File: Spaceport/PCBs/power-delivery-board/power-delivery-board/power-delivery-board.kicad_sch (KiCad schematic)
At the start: 40 parts, among them J1 Conn_01x07_Pin, U1 ADP5033ACBZ-5-R7, U2 TPS610986DSER, U3 TPS610986DSER

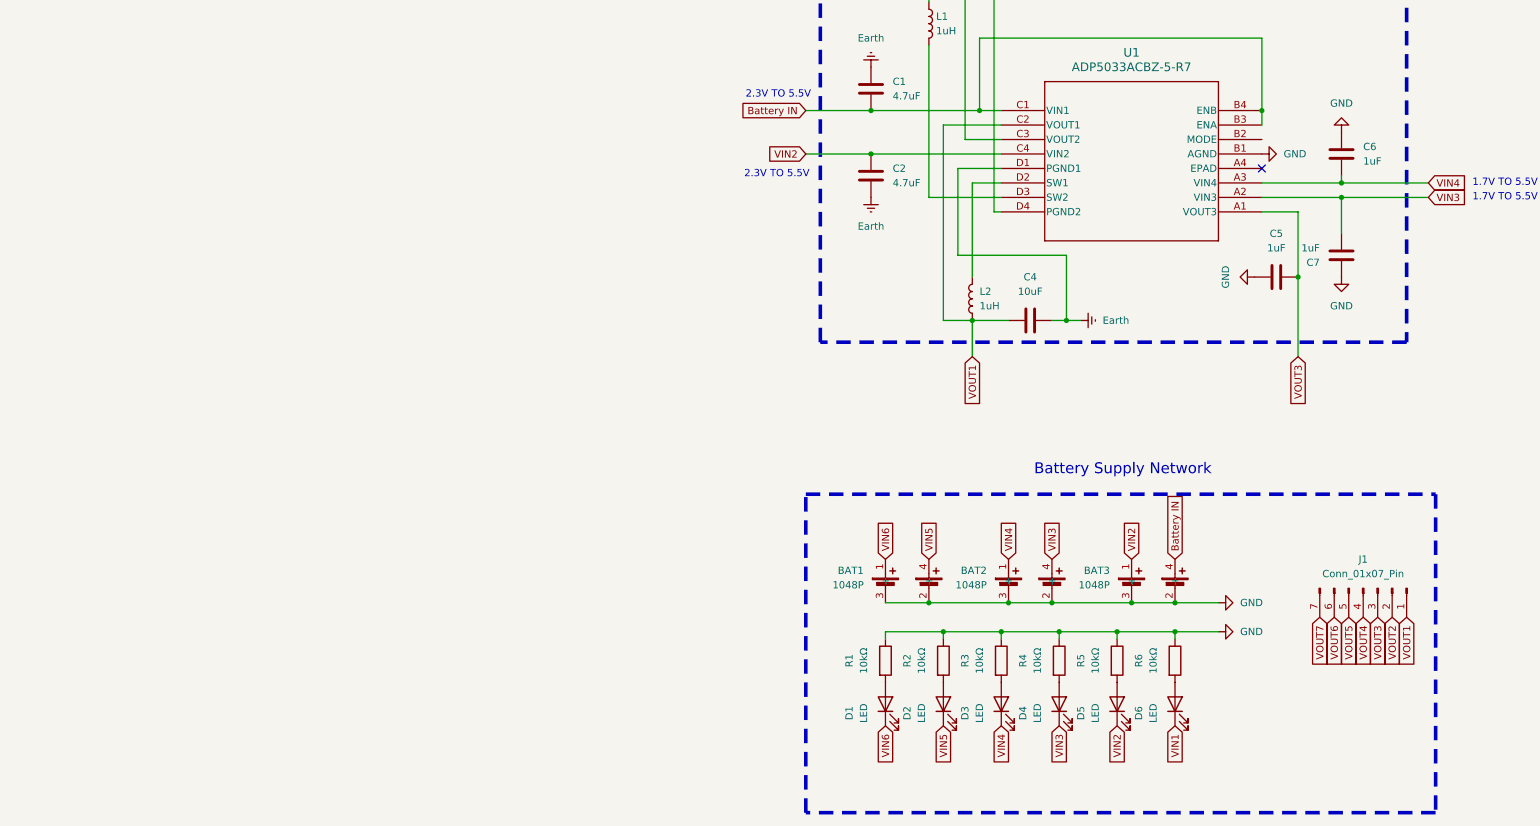
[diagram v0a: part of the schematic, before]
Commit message: Housekeeping File Updates
- Removed extra PCB file that somehow got onto the repo
- Updated PCB file with footprints
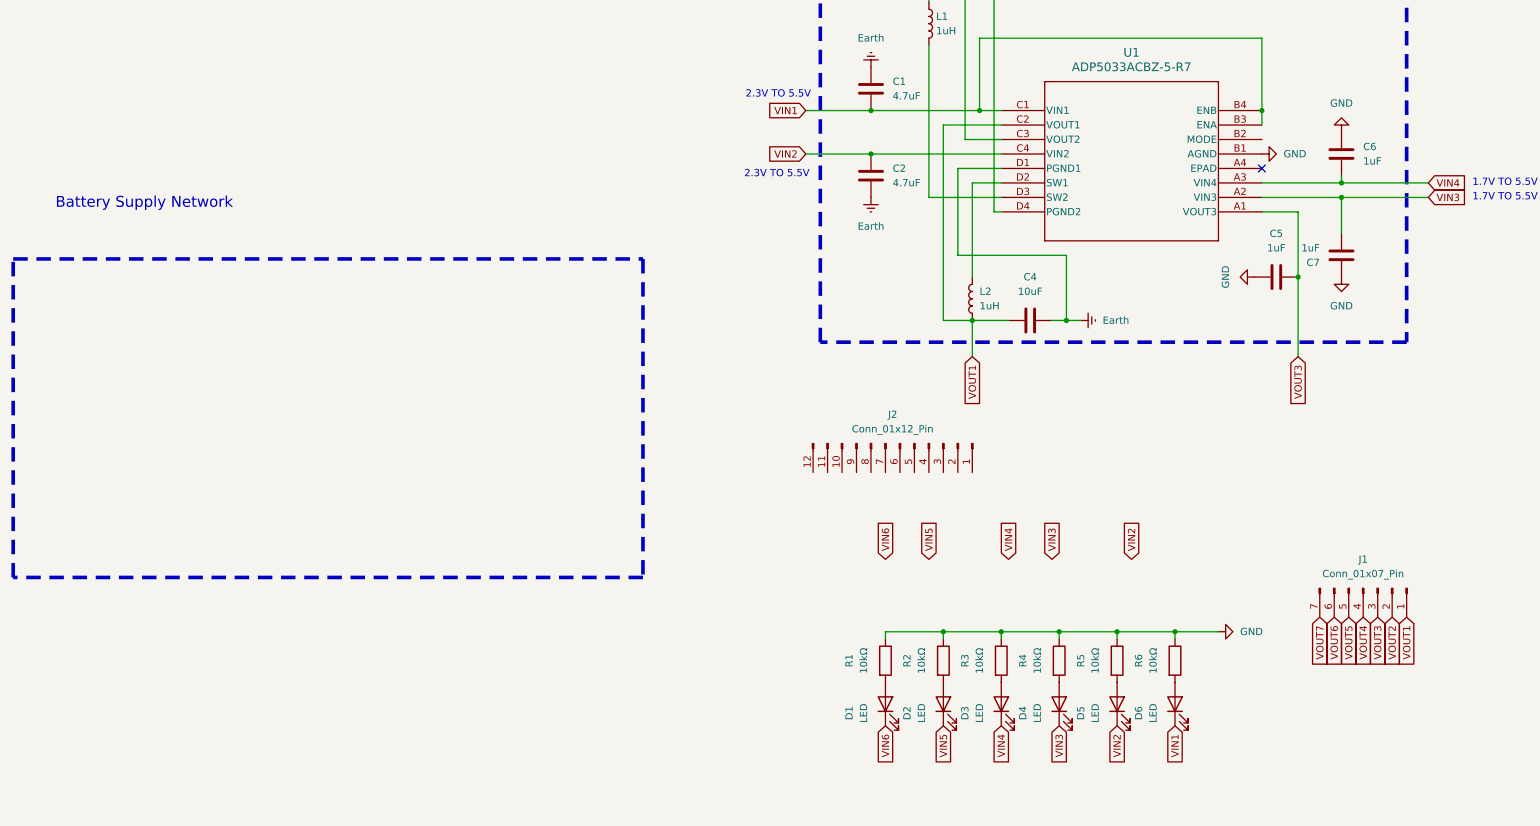
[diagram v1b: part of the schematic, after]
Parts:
- removed BAT1, BAT2, BAT3: 1048P, Avionics:BAT_1048P, symbol Avionics (1):1048P
- added J2: Conn_01x12_Pin, symbol Connector:Conn_01x12_Pin
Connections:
- net Battery IN is gone; now on net VIN1: C1.1, U1.B3 (ENA), U1.B4 (ENB), U1.C1 (VIN1)

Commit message: Add USB and 5V / 3A Topology
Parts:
- removed J2: Conn_01x12_Pin, symbol Connector:Conn_01x12_Pin
- added C10, C11, C12, C13: C, symbol Device:C
- added C8: 1uF, Capacitor_SMD:C_0805_2012Metric, symbol Device:C
- added C9: 4.7uF, symbol Device:C
- added D7, D8: LED, symbol Device:LED
- added J2: Conn_02x06_Row_Letter_Last, symbol Connector_Generic:Conn_02x06_Row_Letter_Last
- added L5: 2.2uH, symbol Device:L
- added P1: USB_C_Plug_USB2.0, symbol Connector:USB_C_Plug_USB2.0
- added R10, R9: 10kΩ, Resistor_SMD:R_0805_2012Metric, symbol Device:R
- added R11: 187kΩ, symbol Device:R
- added R12: 1MΩ, symbol Device:R
- added R13: R, symbol Device:R
- added R7: 1kΩ, symbol Device:R
- added R8: 5kΩ, symbol Device:R
- added U4: USBLC6-2P6, Package_TO_SOT_SMD:SOT-666, symbol Power_Protection:USBLC6-2P6
- added U4: BQ25185DLHR, WSON10_DLH_TEX, symbol Avionics (1):BQ25185DLHR
- added U5: LT8609AEDDM-5#TRPBF, SON50P300X300X85-11N-D, symbol Avionics (1):LT8609AEDDM-5#TRPBF
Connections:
- net GND: now also C12.1, C13.2, C8.1, C9.2, J2.1b (Pin_1b), J2.2b (Pin_2b), J2.3b (Pin_3b), J2.4b (Pin_4b), J2.5b (Pin_5b), J2.6b (Pin_6b), P1.A1 (GND), P1.A12 (GND), P1.B1 (GND), P1.B12 (GND), R10.1, R11.1, R13.2, R7.2, R8.2, R9.1, U4.2 (GND), U4.4 (/CE), U4.5 (GND), U5.11 (GND)
- net VIN1: now also J2.1a (Pin_1a)
- net VIN2: now also J2.2a (Pin_2a)
- net VIN3: now also J2.3a (Pin_3a)
- net VIN4: now also J2.4a (Pin_4a)
- net VIN5: now also J2.5a (Pin_5a)
- net VIN6: now also J2.6a (Pin_6a)
- new net: D7.2 (A), R9.2
- new net: P1.A7 (D-), U4.1 (I/O1)
- new net: P1.A6 (D+), U4.3 (I/O2)
- new net: R13.1, U5.4 (RT)
- new net: C13.1, U5.3 (INTVCC)
- new net: R8.1, U4.7 (ILIM/VSET)
- new net: D8.2 (A), R10.2
- new net: C10.2, U5.1 (BST)
- new net: C10.1, L5.2, U5.2 (SW)
- new net: R7.1, U4.8 (ISET)
- new net BAT+: U4.2 (BAT)
- new net D+: U4.4 (I/O2)
- new net D-: U4.6 (I/O1)
- new net FB: C11.1, R11.2, R12.1, U5.6 (FB)
- new net STAT1: D7.1 (K), U4.9 (STAT1)
- new net STAT2: D8.1 (K), U4.3 (STAT2)
- new net VBUS: C8.2, P1.A4 (VBUS), P1.A9 (VBUS), P1.B4 (VBUS), P1.B9 (VBUS), U4.10 (IN), U4.5 (VBUS)
- new net VIN7: C9.1, U5.9 (VIN)
- new net VOUT8: C11.2, C12.2, L5.1, R12.2
- no-connect marks 3 -> 8
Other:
- note added: "6V TO 40V"
- note added: "INPUT / OUTPUT"
- note added: "SOURCE THREE"
- note added: "STATUS LEDs"
- note added: "VOUT 8 5V 3A"
- note removed: "Battery Supply Network"
- moved on the sheet: C1, C2, C3, C4, C5, C6, C7, CBAT1, CBAT2, CIN1, CIN2, COUT1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

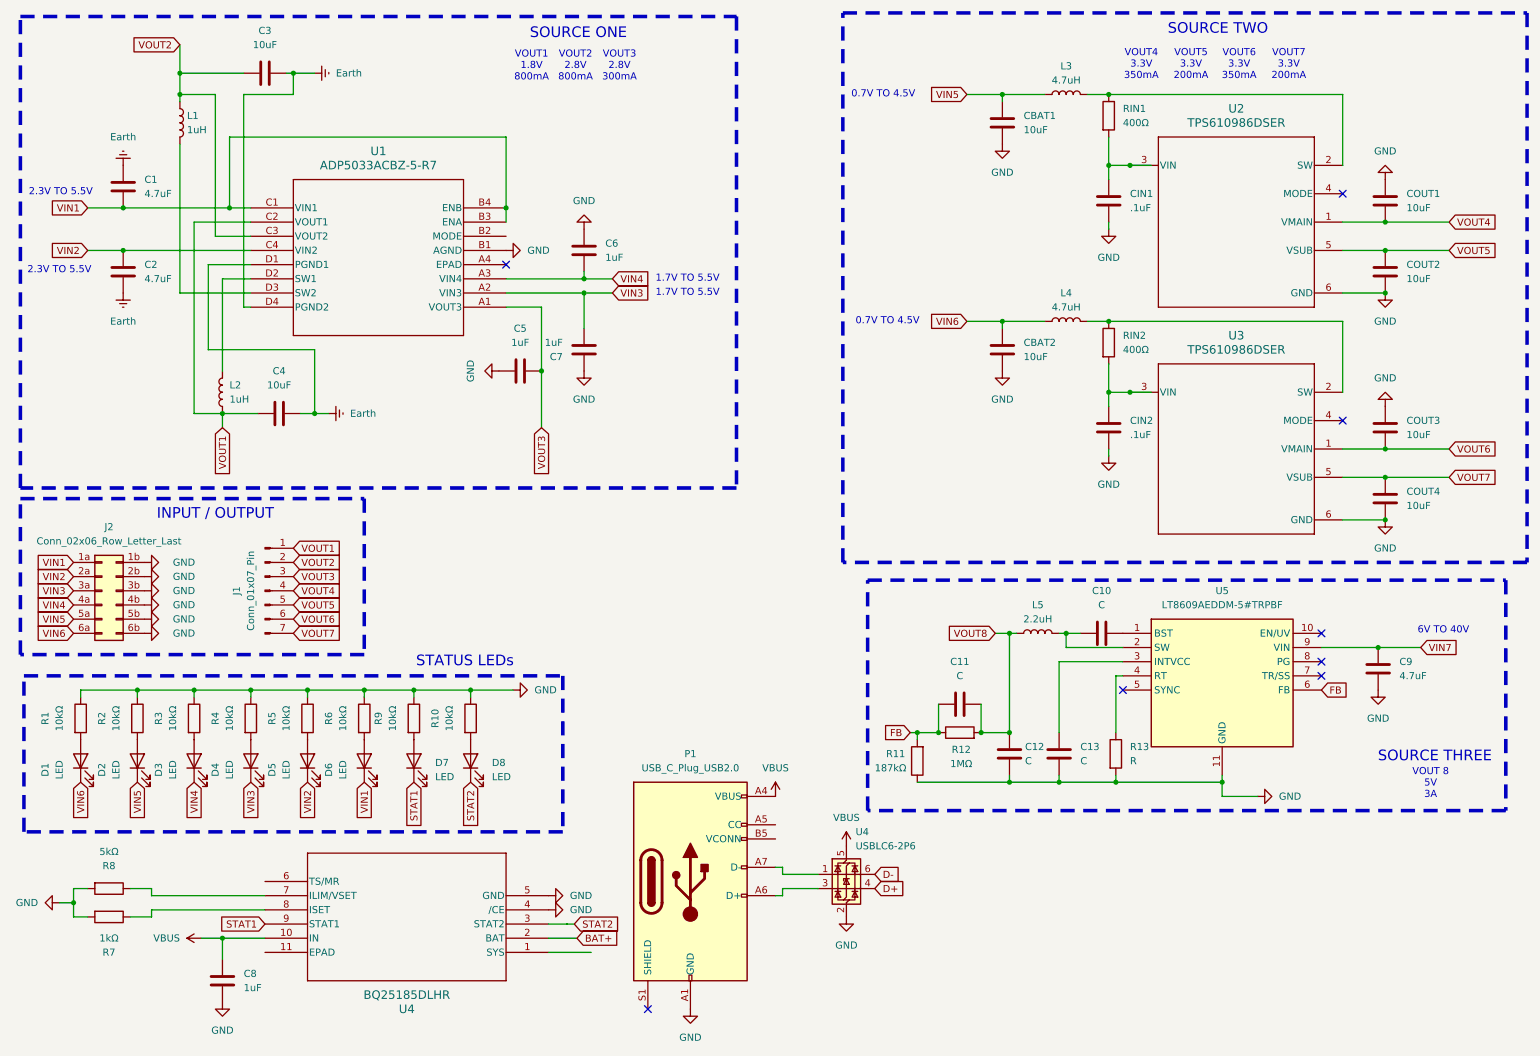
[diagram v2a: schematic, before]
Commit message: Schematic Updates. NOTE: ERC Fails
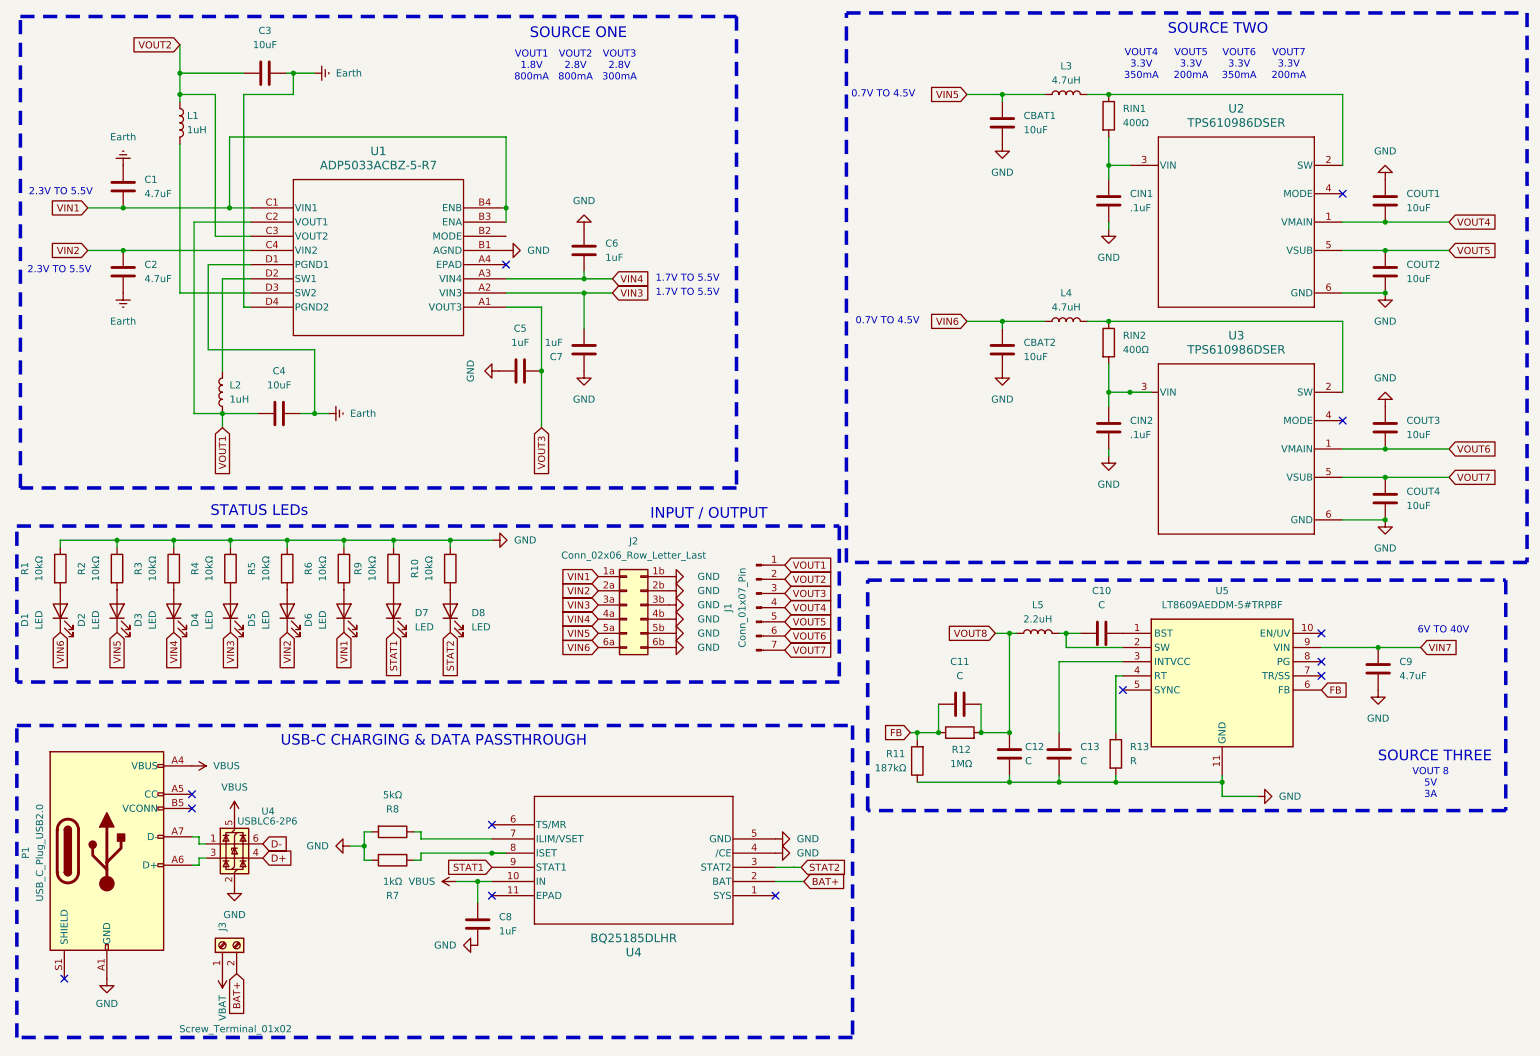
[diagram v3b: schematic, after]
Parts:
- added J3: Screw_Terminal_01x02, symbol Connector:Screw_Terminal_01x02
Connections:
- net BAT+: now also J3.2 (Pin_2)
- new net VBAT: J3.1 (Pin_1)
- no-connect marks 8 -> 13
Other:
- note added: "USB-C CHARGING & DATA PASSTHROUGH"
- moved on the sheet: C8, D1, D2, D3, D4, D5, D6, D7, D8, J1, J2, P1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
